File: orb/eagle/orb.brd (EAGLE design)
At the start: 80.8 x 80.8 mm, 22 parts, among them J1 MICRO USB, Q1 CRYSTAL, T1 DMG2302U, T2 DMG2302U, T3 DMG2302U, U1 PRTR5V0U2X, U2 ATTINY2313

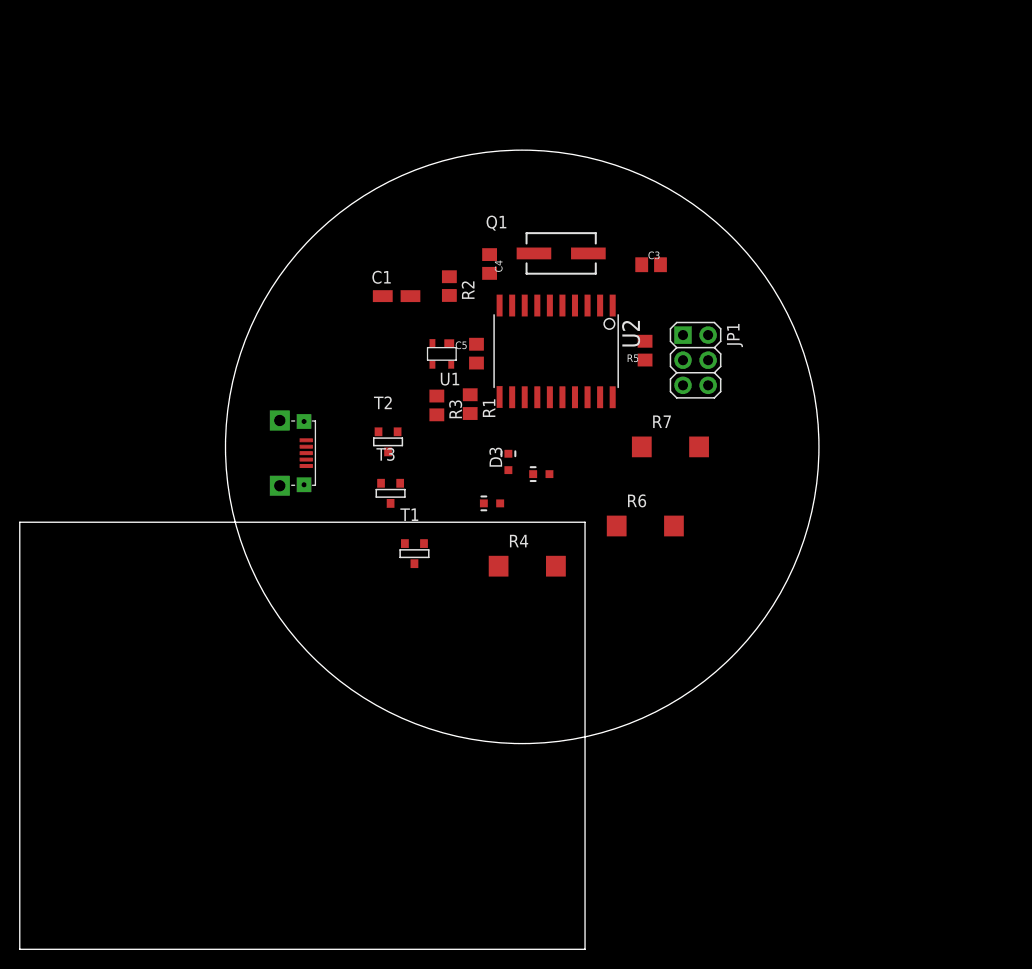
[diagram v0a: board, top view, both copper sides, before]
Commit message: First iteration of layout. Work in progress.
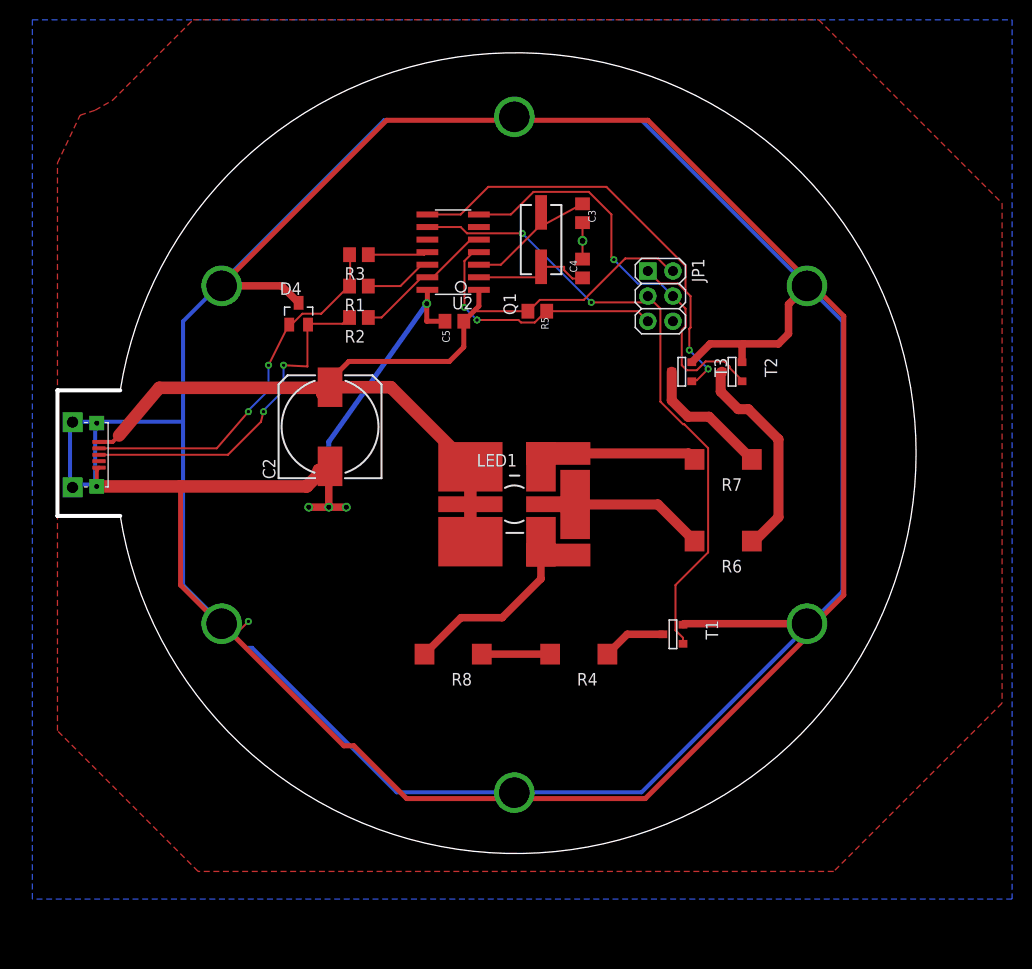
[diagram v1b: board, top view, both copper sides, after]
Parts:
- removed C1: 47U, rcl:CT3216
- removed D1: GREEN, arm-pro-mini:LED0603
- removed D2: RED, arm-pro-mini:LED0603
- removed D3: BLUE, arm-pro-mini:LED0603
- removed U1: PRTR5V0U2X, arm-pro-mini:SOT143B
- added C2: 1000U 10V, rcl:153CLV-1010
- added D4: AZ23C3V6, orb:SOT23
- added LED1: OVSTRGBBCR4, orb:OVSTRGBBCR4
- added R8: ?? 1W, rcl:R2512W
- added U$1, U$12, U$2, U$3, U$4, U$5: MOUNTING_HOLE, orb:MOUNTING_HOLE
- Q1: value CRYSTAL -> 12MHZ
- U2: value ATTINY2313 -> ATINY44A; device orb:ATTINY2313 -> orb:SOIC14
- moved T2 35.5 mm to (72.0, 58.4), turned to 270 degrees
- moved T3 31.9 mm to (66.9, 58.4), turned to 270 degrees
- moved T1 27.4 mm to (66.0, 31.9), turned to 270 degrees
- moved J1 21.0 mm to (5.33, 50.0)
- moved R3 17.2 mm to (34.3, 70.2), turned to 180 degrees
- moved R1 16.4 mm to (34.3, 67.1), turned to 180 degrees
- moved U2 14.5 mm to (43.8, 70.5), turned to 90 degrees
- moved R5 11.6 mm to (52.3, 64.5), turned to 180 degrees
- moved R4 10.3 mm to (56.5, 29.8), turned to 180 degrees
- moved R2 9.68 mm to (34.3, 63.9), turned to 180 degrees
- moved C4 9.41 mm to (56.9, 68.8), turned to 90 degrees
- moved C3 8.67 mm to (56.9, 74.4), turned to 270 degrees
- moved R6 8.02 mm to (71.1, 41.3), turned to 180 degrees
- moved JP1 7.39 mm to (64.8, 66.0)
- moved R7 5.48 mm to (71.1, 49.5), turned to 180 degrees
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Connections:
- removed net BLUE: T3.3, U2.16
- removed net GREEN: T2.3, U2.12
- removed net MISO: JP1.1, U2.18
- removed net MOSI: JP1.4
- removed net N$11: D1.C, R6.2
- removed net N$12: D3.C, R7.2
- removed net RED: T1.3, U2.14
- removed net SCK: JP1.3, U2.19
- new net MISO/GREEN: JP1.1, T3.3, U2.8
- new net MOSI/RED: JP1.4, T2.3, U2.7
- new net N$8: LED1.5, LED1.5@1, R6.2
- new net N$9: LED1.4, LED1.4@1, R7.2
- new net SCK/BLUE: JP1.3, T1.3, U2.9
- net +5V: now also C2.+, LED1.1, LED1.2, LED1.3, U2.1; no longer C1.+, D1.A, D2.A, D3.A, U1.4, U2.20
- net DM: now also U2.12; no longer U2.7
- net DP: now also U2.13, U2.5; no longer U2.6
- net GND: now also C2.-, D4.3, U$1.P1, U$12.P1, U$2.P1, U$3.P1, U$4.P1, U$5.P1, U2.14; no longer C1.-, U1.1, U2.10
- net N$1: now also U2.3; no longer U2.4
- net N$3: now also U2.2; no longer U2.5
- net N$4: now also R4.2, R8.1; no longer U2.17
- net N$5: now also D4.1; no longer U1.3
- net N$6: now also D4.2; no longer U1.2
- net N$7: now also LED1.6, LED1.6@1, R8.2; no longer D2.C, R4.2
- net RESET: now also U2.4; no longer U2.1
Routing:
- net GND: track 0.00 -> 558.8 mm, vias 0 -> 6
- net +5V: track 0.00 -> 97.9 mm
- net SCK/BLUE: track 0.00 -> 66.2 mm, vias 0 -> 2
- net MISO/GREEN: track 0.00 -> 48.9 mm, vias 0 -> 2
- net MOSI/RED: track 0.00 -> 42.8 mm, vias 0 -> 1
- net N$5: track 0.00 -> 38.0 mm, vias 0 -> 2
- net N$6: track 0.00 -> 35.5 mm, vias 0 -> 2
- net RESET: track 0.00 -> 26.6 mm, vias 0 -> 2
- net N$14: track 0.00 -> 21.5 mm
- net N$7: track 0.00 -> 18.7 mm
- net DP: track 0.00 -> 14.4 mm
- net N$1: track 0.00 -> 14.3 mm
- net N$9: track 0.00 -> 14.0 mm
- net N$8: track 0.00 -> 13.6 mm
- net N$15: track 0.00 -> 13.5 mm
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- added copper zone on layer 1, net GND
- added copper zone on layer 16, net GND
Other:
- board size 80.8 x 80.8 mm -> 86.8 x 80.9 mm
